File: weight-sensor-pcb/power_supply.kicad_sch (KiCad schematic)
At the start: 7 parts, among them U1 TPS54202DDC

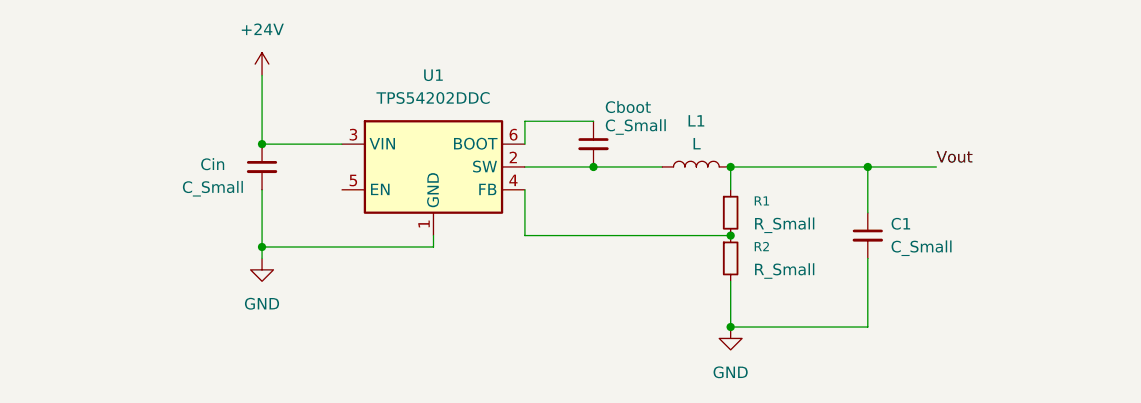
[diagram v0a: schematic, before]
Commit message: finish converter schematic
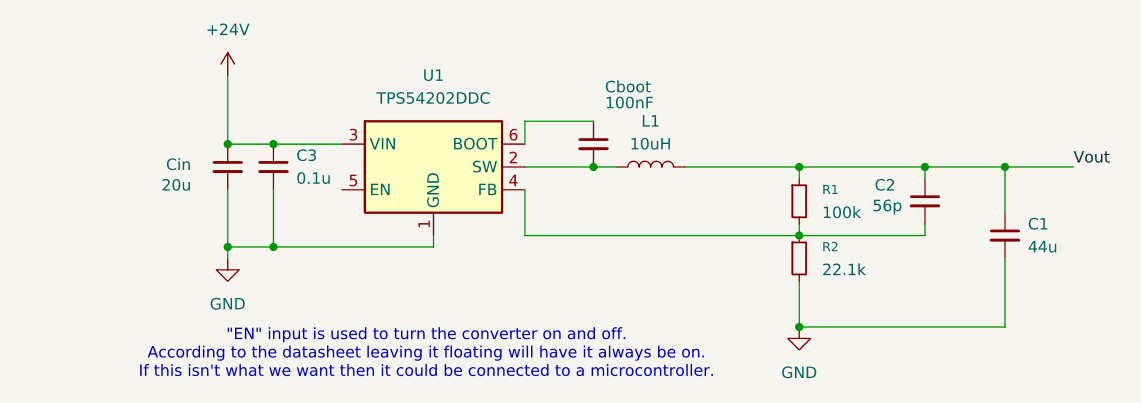
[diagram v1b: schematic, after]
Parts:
- added C2: 56p, symbol Device:C_Small
- added C3: 0.1u, symbol Device:C_Small
- C1: value C_Small -> 44u
- Cboot: value C_Small -> 100nF
- Cin: value C_Small -> 20u
- L1: value L -> 10uH
- R1: value R_Small -> 100k
- R2: value R_Small -> 22.1k
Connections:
- net +24V: now also C3.1
- net GND: now also C3.2
- net Vout: now also C2.1
- net at R1.2, R2.1, U1.4 (FB): now also C2.2
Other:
- note added: ""EN" input is used to turn the converter on and off. According to the datasheet leaving it floating will have it always be on. If this isn't what we want then it could be connected to a microcontroller."
- moved on the sheet: C1, Cin, L1, R1, R2
